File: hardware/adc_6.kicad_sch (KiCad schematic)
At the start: 12 parts, among them J5 Conn_01x04, U5 ADS122C04IPW

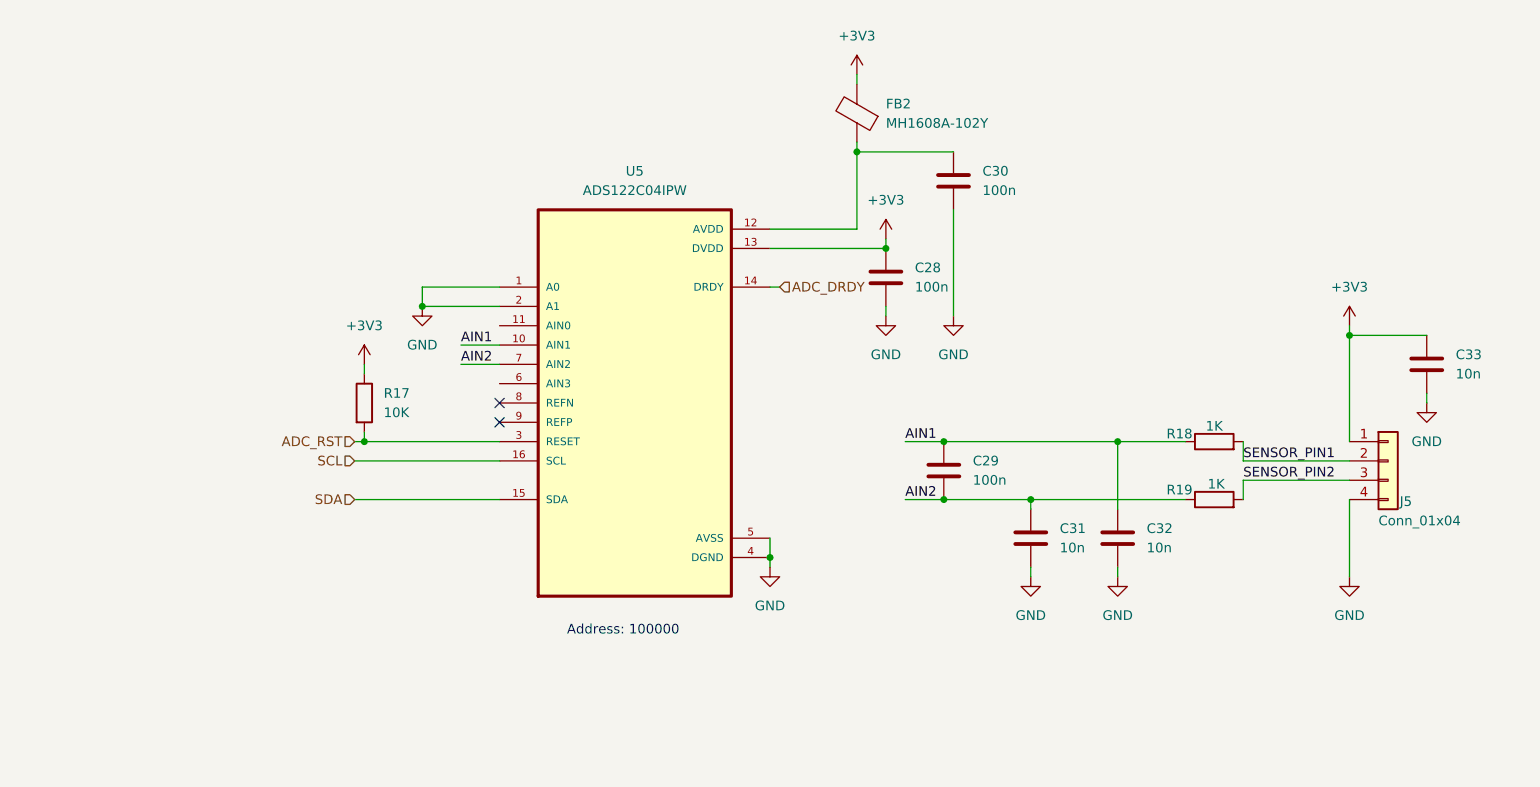
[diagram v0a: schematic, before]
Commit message: Organize schematic
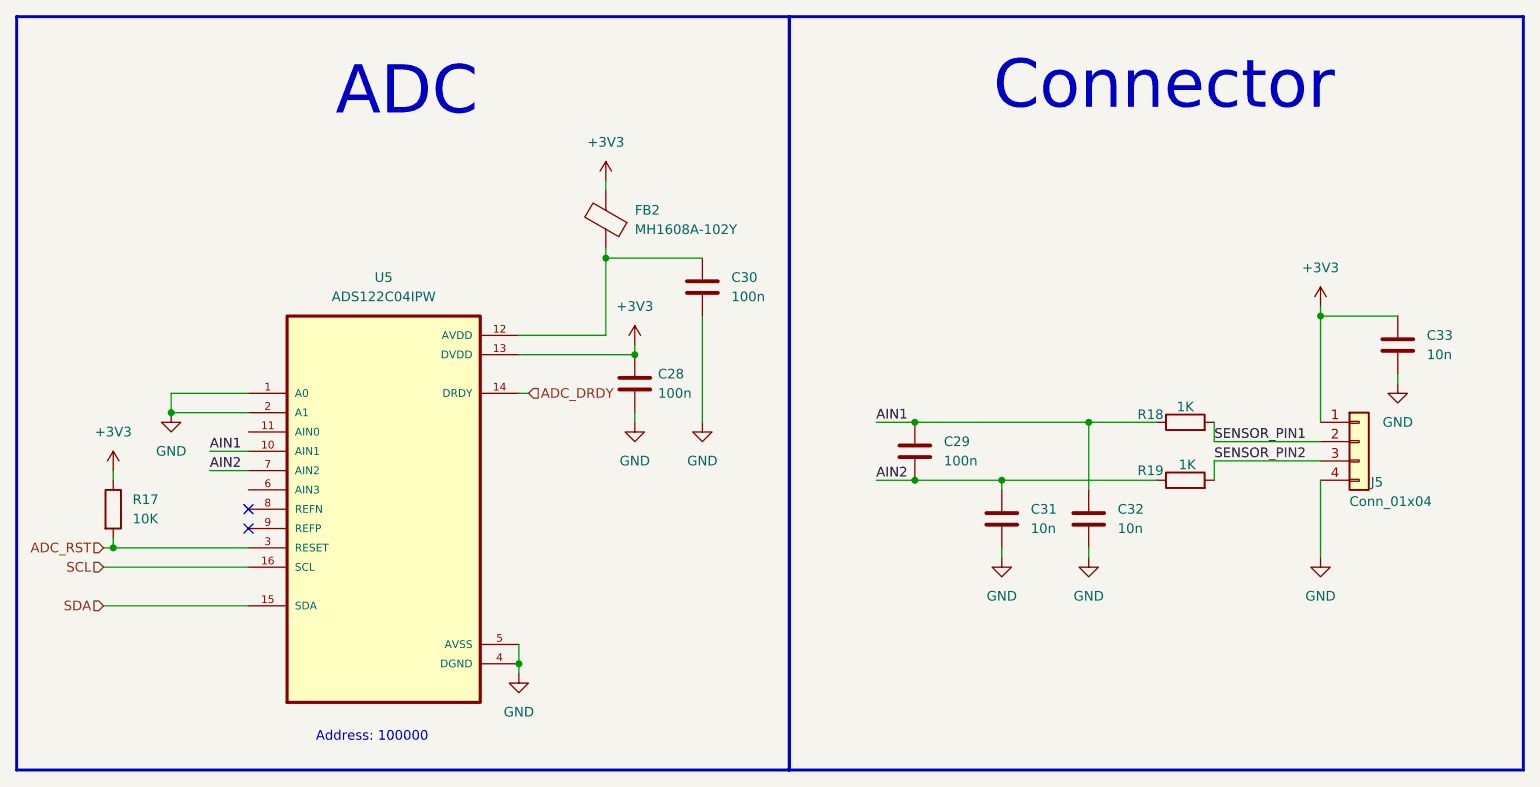
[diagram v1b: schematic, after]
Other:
- note added: "ADC"
- note added: "Connector"
- moved on the sheet: C28, C29, C30, C31, C32, C33, FB2, J5, R17, R18, R19, U5
